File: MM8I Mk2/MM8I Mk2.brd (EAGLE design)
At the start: 160 x 100 mm, 14 parts, among them U1 CY14B104M, U2 SN74LVC16T245DGVR

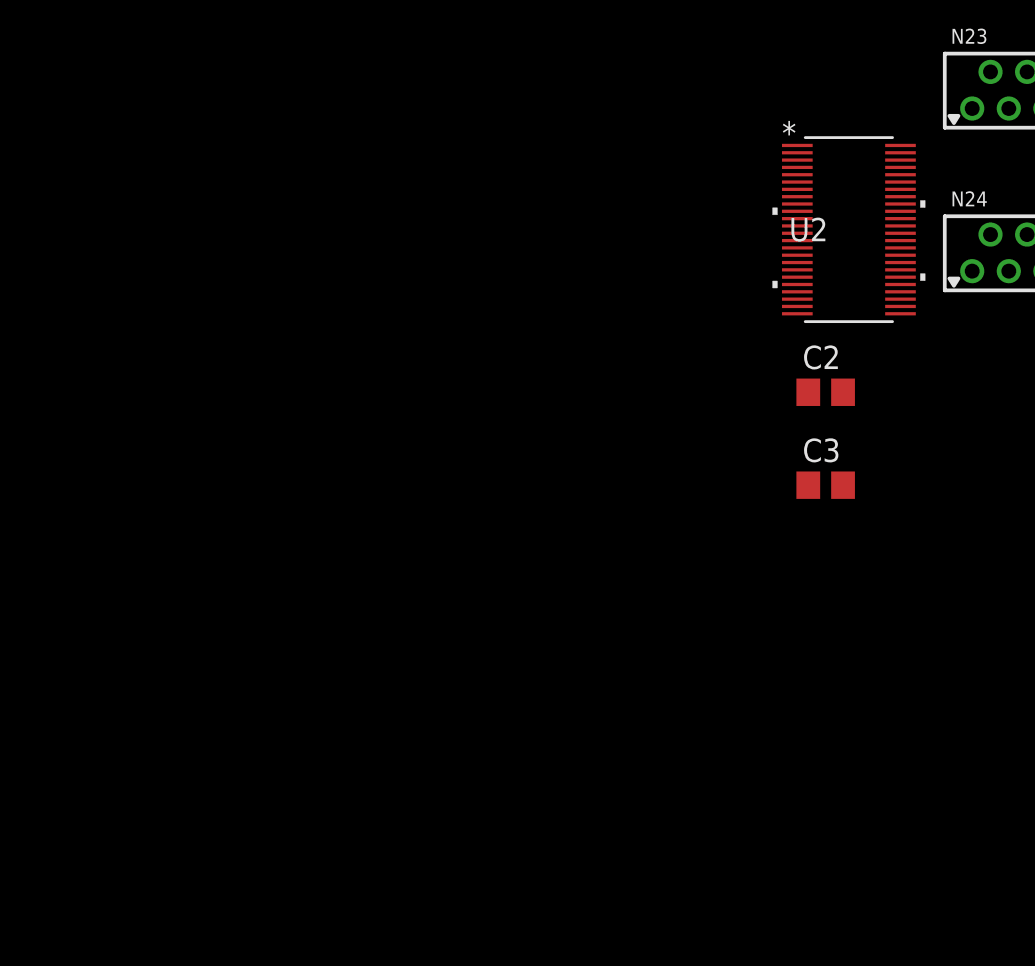
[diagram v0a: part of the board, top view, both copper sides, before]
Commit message: Progress on MM8I Mk2
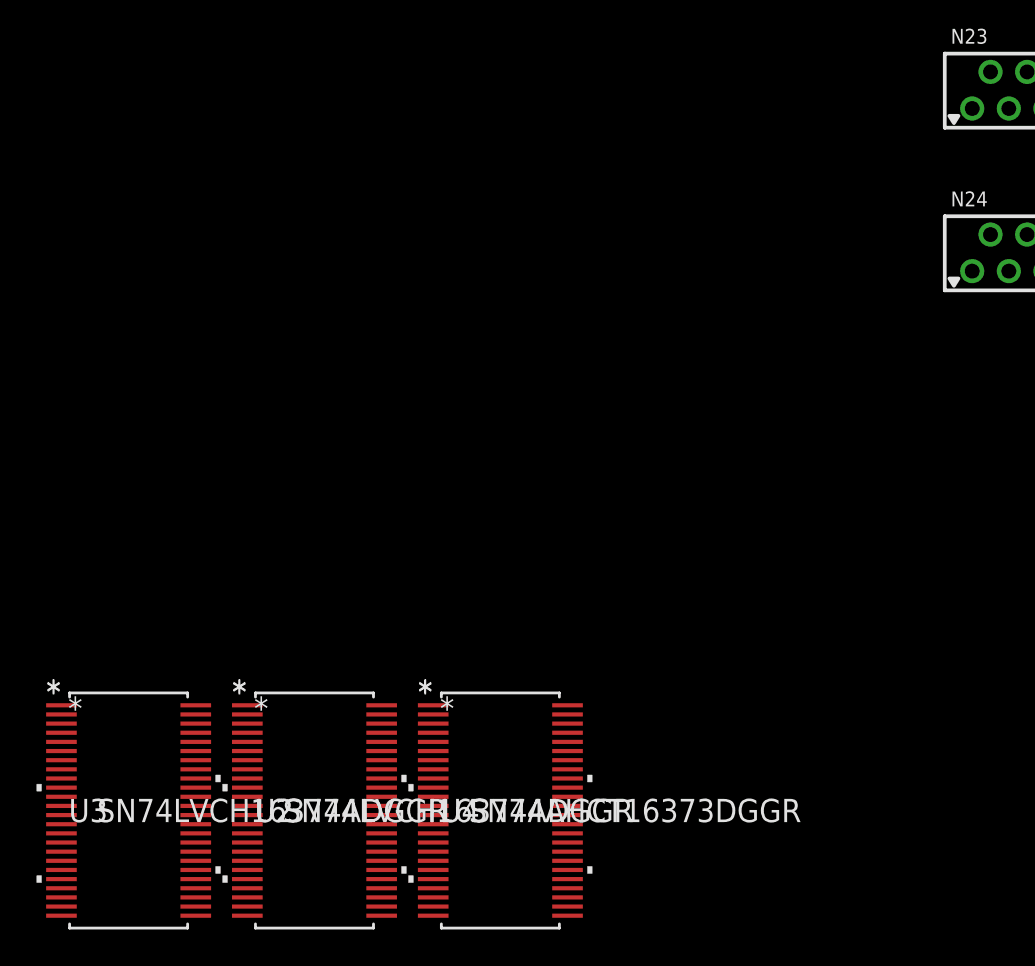
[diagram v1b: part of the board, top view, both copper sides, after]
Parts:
- removed C2, C3: (no value), rcl:C0805
- added U3: SN74LVCH16374ADGGR, MM24I:DGG48
- added U4: SN74AHCT16373DGGR, MM24I:DGG48
- U2: value SN74LVC16T245DGVR -> SN74LVCH16374ADGGR; device MM24I:DGV48 -> MM24I:DGG48
- moved U2 43.1 mm to (-67.3, -127.0)
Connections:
- removed net N$18: U2.2
- removed net N$19: U2.3
- removed net N$20: U2.5
- removed net N$21: U2.6
- removed net N$22: U2.8
- removed net N$23: U2.9
- removed net N$24: U2.11
- removed net N$25: U2.12
- removed net N$26: U2.13
- removed net N$27: U2.14
- removed net N$28: U2.16
- removed net N$29: U2.17
- new net N$32: U1.3, U3.13
- new net N$33: U1.4, U3.14
- new net N$34: U1.6, U3.17
- new net N$36: U1.7, U3.19
- new net N$37: U1.20, U3.20
- new net N$38: U1.21, U3.22
- new net N$39: U1.22, U3.23
- new net N$40: U1.24, U3.3
- new net N$41: U1.31, U3.5
- new net N$42: U1.32, U3.6
- new net N$43: U1.33, U3.8
- new net N$44: U1.34, U3.9
- new net N$45: U1.35, U3.11
- net !WE: no longer U2.1, U2.24
- net +5V: now also U4.18, U4.31, U4.42, U4.7; no longer C3.2
- net GND: now also R1.1, R2.1, R3.1, R4.1, U1.47, U1.48, U1.50, U1.51, U1.52, U1.8, U2.1, U2.24, U3.1, U3.10, U3.15, U3.21, U3.24, U3.26, U3.28, U3.34, U3.39, U3.4, U3.45, U4.1, U4.10, U4.15, U4.21, U4.24, U4.26, U4.27, U4.28, U4.29, U4.30, U4.34, U4.39, U4.4, U4.45; no longer R1.2, R2.2, R3.2, R4.2, U2.19, U2.20, U2.22, U2.23, U2.25, U2.48
- net MCS-MEM-00-H: now also U4.2
- net MCS-MEM-01-H: now also U4.3
- net MCS-MEM-02-H: now also U4.5
- net MCS-MEM-03-H: now also U4.6
- net MCS-MEM-04-H: now also U4.8
- net MCS-MEM-05-H: now also U4.9
- net MCS-MEM-06-H: now also U4.11
- net MCS-MEM-07-H: now also U4.12
- net MCS-MEM-08-H: now also U4.13
- net MCS-MEM-09-H: now also U4.14
- net MCS-MEM-10-H: now also U4.16
- net MCS-MEM-11-H: now also U4.17
- net MXB-BMA-00-H: now also U3.47
- net MXB-BMA-01-H: now also U3.46
- net MXB-BMA-02-H: now also U3.44
- net MXB-BMA-03-H: now also U3.43
- net MXB-BMA-04-H: now also U3.41
- net MXB-BMA-05-H: now also U3.40
- net MXB-BMA-06-H: now also U3.38
- net MXB-BMA-07-H: now also U3.37
- net MXB-BMA-08-H: now also U3.36
- net MXB-BMA-09-H: now also U3.35
- net MXB-BMA-10-H: now also U3.33
- net MXB-BMA-11-H: now also U3.32
- net MXB-MCBMB-00-H: now also U2.47
- net MXB-MCBMB-01-H: now also U2.46
- net MXB-MCBMB-02-H: now also U2.44
- net MXB-MCBMB-03-H: now also U2.43
- net MXB-MCBMB-04-H: now also U2.41
- net MXB-MCBMB-05-H: now also U2.40
- net MXB-MCBMB-06-H: now also U2.38
- net MXB-MCBMB-07-H: now also U2.37
- net MXB-MCBMB-08-H: now also U2.36
- net MXB-MCBMB-09-H: now also U2.35
- net MXB-MCBMB-10-H: now also U2.33
- net MXB-MCBMB-11-H: now also U2.32
- net MXF-EA-00-H: now also U3.30
- net MXF-EA-01-H: now also U3.29
- net MXF-EA-02-H: now also U3.27
- net N$10: now also R2.2, U1.45; no longer R4.1, U1.46
- net N$11: now also U2.22, U4.38; no longer U2.38
- net N$12: now also R3.2, U1.44; no longer R1.1, U1.43
- net N$13: now also U2.23, U4.37; no longer U2.37
- net N$14: now also U2.2, U4.36; no longer U2.36
- net N$15: now also U2.3, U4.35; no longer U2.35
- net N$16: now also U2.5, U4.33; no longer U2.33
- net N$17: now also U2.6, U4.32; no longer U2.32
- net N$2: now also U2.13, U4.47; no longer U2.47
- net N$3: now also U2.14, U4.46; no longer U2.46
- net N$30: now also U1.23, U3.2; no longer C3.1, U2.18, U2.7
- net N$31: now also U1.5, U3.16; no longer C2.1, U2.31, U2.42
- net N$4: now also U2.16, U4.44; no longer U2.44
- net N$5: now also U2.17, U4.43; no longer U2.43
- net N$6: now also U2.19, U4.41; no longer U2.41
- net N$7: now also U2.20, U4.40; no longer U2.40
- net N$8: now also R4.2, U1.43; no longer R2.1, U1.44
- net N$9: now also R1.2, U1.46; no longer R3.1, U1.45
- net VCC: now also U2.18, U2.31, U2.42, U2.7, U3.18, U3.31, U3.42, U3.7; no longer C2.2
